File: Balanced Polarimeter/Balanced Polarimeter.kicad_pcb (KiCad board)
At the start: 2 copper layers, 57.5 x 40 mm, 16 parts, among them IC1 OP27, J1 73100-0105, Q1 MMPQ3904, Q2 MMPQ3904, U1 ADA4898-1YRDZ, U2 ADA4898-1YRDZ

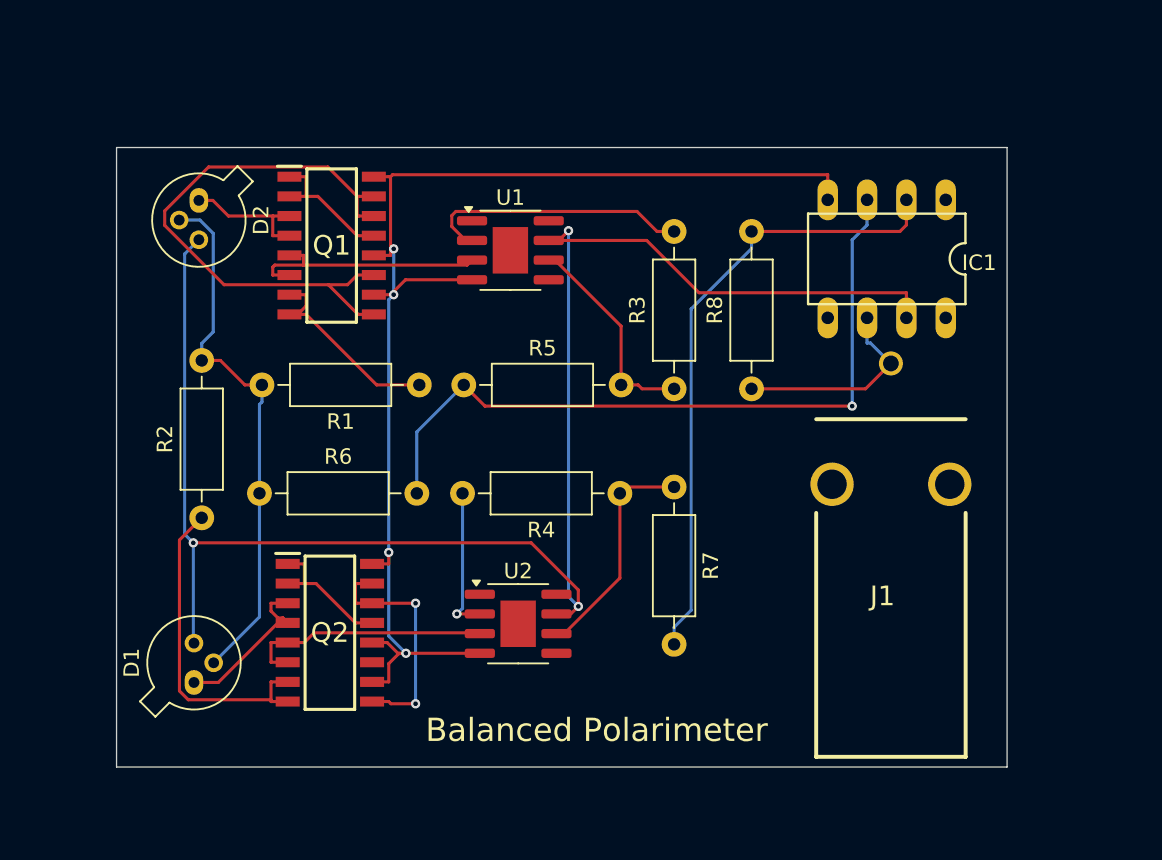
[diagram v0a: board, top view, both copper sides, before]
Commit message: Updates
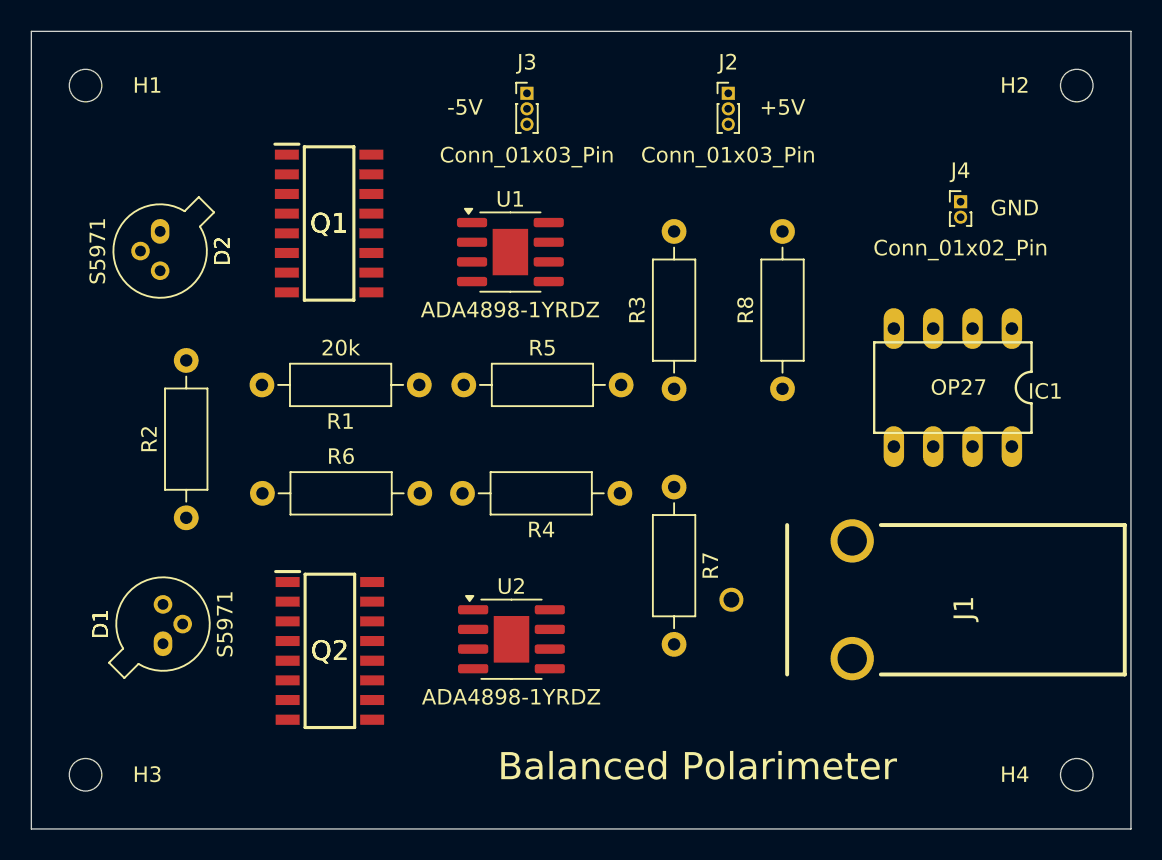
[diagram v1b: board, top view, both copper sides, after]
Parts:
- added H1: MountingHole, MountingHole:MountingHole_2.1mm, F.Cu at (125.5, 60.0)
- added H2: MountingHole, MountingHole:MountingHole_2.1mm, F.Cu at (189.5, 60.0)
- added H3: MountingHole, MountingHole:MountingHole_2.1mm, F.Cu at (125.5, 104.5)
- added H4: MountingHole, MountingHole:MountingHole_2.1mm, F.Cu at (189.5, 104.5)
- added J2: Conn_01x03_Pin, Connector_PinHeader_1.00mm:PinHeader_1x03_P1.00mm_Vertical, F.Cu at (167.0, 60.5)
- added J3: Conn_01x03_Pin, Connector_PinHeader_1.00mm:PinHeader_1x03_P1.00mm_Vertical, F.Cu at (154.0, 60.5)
- added J4: Conn_01x02_Pin, Connector_PinHeader_1.00mm:PinHeader_1x02_P1.00mm_Vertical, F.Cu at (182.0, 67.5)
- moved J1 18.2 mm to (192.6, 93.2), turned to 90 degrees
- moved IC1 9.34 mm to (181.5, 79.5)
- moved D2 3.20 mm to (130.3, 69.4)
- moved D1 3.20 mm to (130.5, 96.0)
- moved R8 2.00 mm to (170.5, 79.6)
- moved Q1 1.43 mm to (141.2, 68.9)
- moved Q2 1.17 mm to (141.3, 96.5)
- moved U2 1.09 mm to (153.0, 95.8)
- moved R2 1.00 mm to (132.0, 87.9)
- moved R6 0.19 mm to (136.9, 86.3)
- moved U1 0.11 mm to (152.9, 70.8)
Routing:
- net +5V: track 107.6 -> 0.00 mm, vias 3 -> 0
- net -5V: track 83.2 -> 0.00 mm, vias 4 -> 0
- net Net-(IC1-Pad3): track 47.6 -> 0.00 mm, vias 1 -> 0
- net Net-(IC1-Pad2): track 40.5 -> 0.00 mm
- net Net-(Q1-BASE_#1): track 37.9 -> 0.00 mm
- net GND: track 34.8 -> 0.00 mm
- net Net-(Q2-COLLECTOR_#4_1): track 21.3 -> 0.00 mm
- net Net-(U1--): track 17.4 -> 0.00 mm
- net Net-(Q1-COLLECTOR_#3_1): track 16.2 -> 0.00 mm
- net Net-(Q2-COLLECTOR_#3_1): track 16.1 -> 0.00 mm
- net Net-(Q2-BASE_#1): track 15.6 -> 0.00 mm, vias 2 -> 0
- net Net-(R4-Pad1): track 14.7 -> 0.00 mm
- net Net-(R3-Pad1): track 13.8 -> 0.00 mm
- net V_out: track 13.4 -> 0.00 mm
- net Net-(Q1-COLLECTOR_#4_1): track 12.8 -> 0.00 mm
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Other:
- board size 57.5 x 40 mm -> 71 x 51.5 mm
- board text added: "+5V"
- board text added: "-5V"
- board text added: "GND"
